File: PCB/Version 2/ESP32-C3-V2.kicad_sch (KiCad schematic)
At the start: 33 parts, among them J3 HCZZ0001-4, Q1 WPM2031-3/TR, SW2 TS-1187A-B-A-B, U1 USB-C-16P-SMD, U3 ESP32-C3, Y1 40MHz_S3240000151040

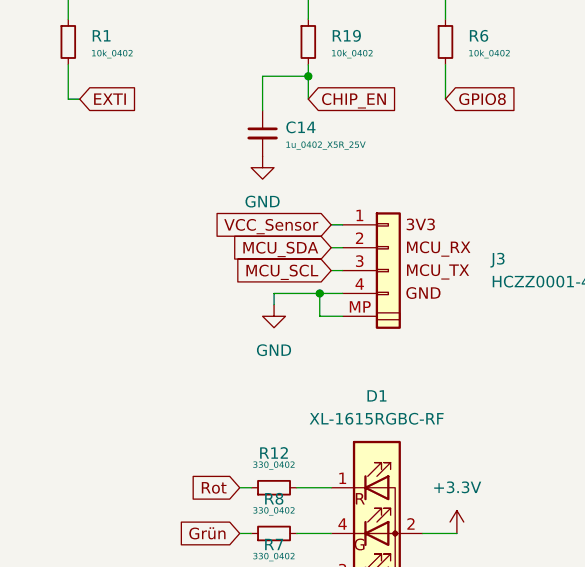
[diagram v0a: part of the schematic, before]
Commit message: neue Bilder, Gerber, PDF
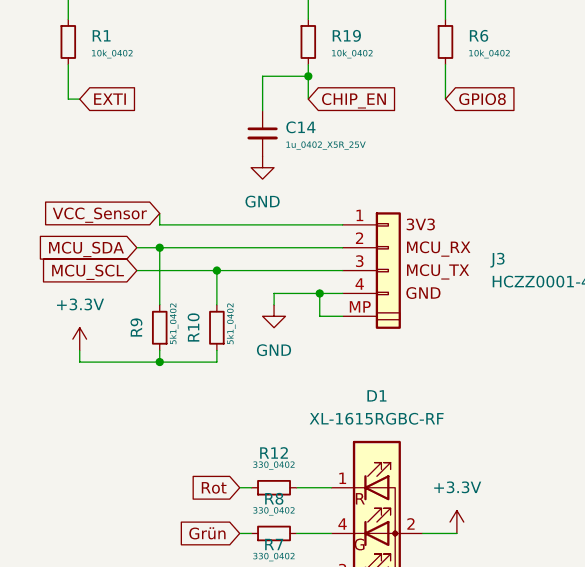
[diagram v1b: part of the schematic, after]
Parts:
- added R10, R9: 5k1_0402, Resistor_SMD:R_0402_1005Metric, symbol resistor_smd_standard:5k1_0402
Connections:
- net +3.3V: now also R10.1, R9.1
- net MCU_SCL: now also R10.2
- net MCU_SDA: now also R9.2

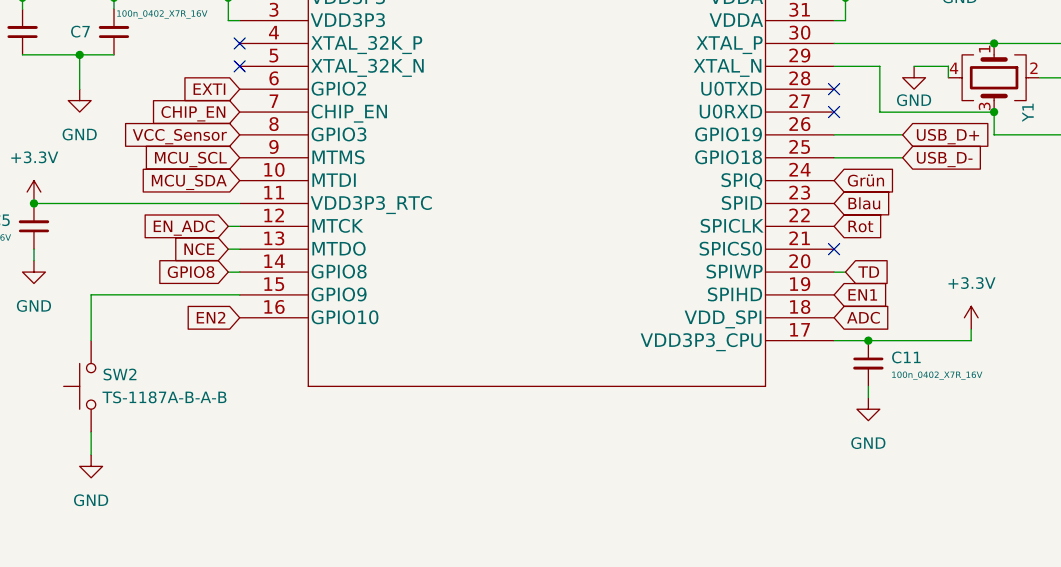
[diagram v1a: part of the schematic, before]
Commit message: Version 2 zur Korrektur fertig
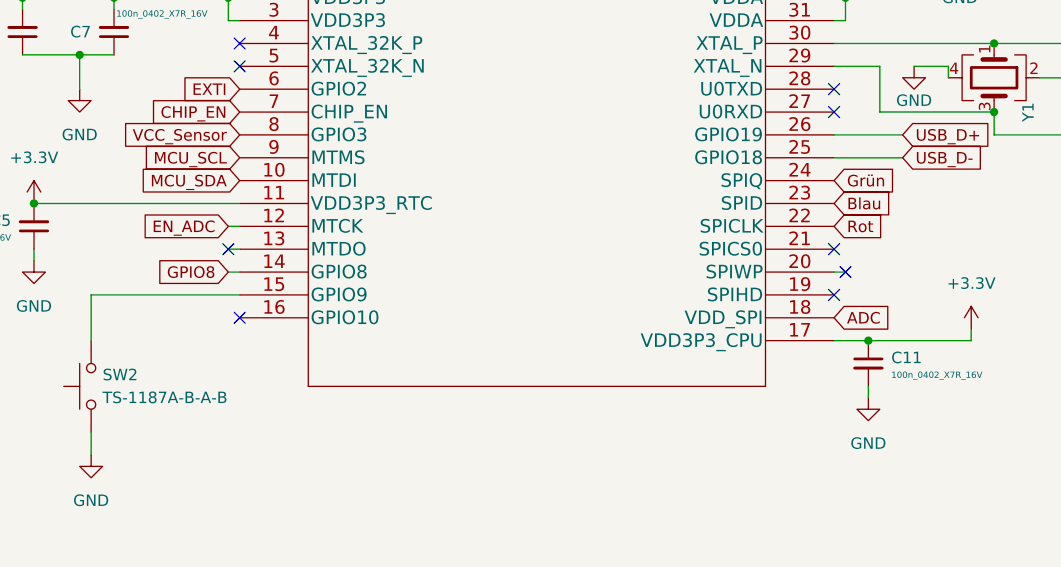
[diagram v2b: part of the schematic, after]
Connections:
- net EN1: no longer names the net of U3.19 (SPIHD)
- net EN2: no longer names the net of U3.16 (GPIO10)
- net NCE: no longer names the net of U3.13 (MTDO)
- net TD: no longer names the net of U3.20 (SPIWP)
- no-connect marks 15 -> 19
